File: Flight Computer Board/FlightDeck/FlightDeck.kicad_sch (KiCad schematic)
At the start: 15 parts, among them SW1 SW_SPDT, U1 STM32F205RBT6

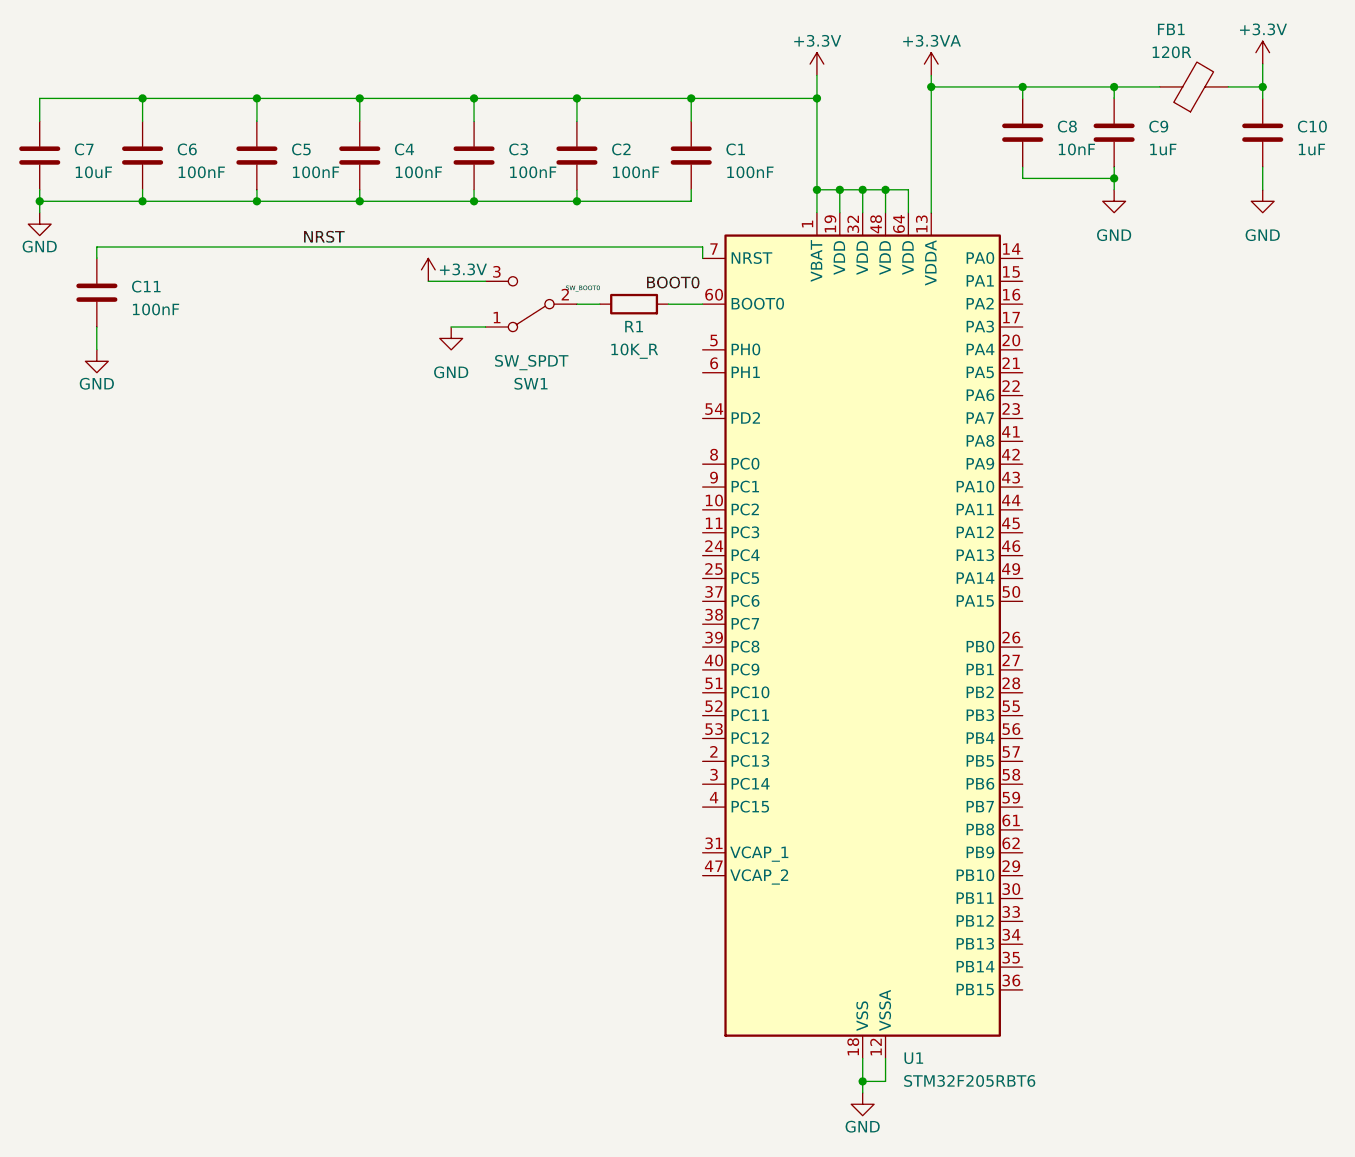
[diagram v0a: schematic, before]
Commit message: fc: init design
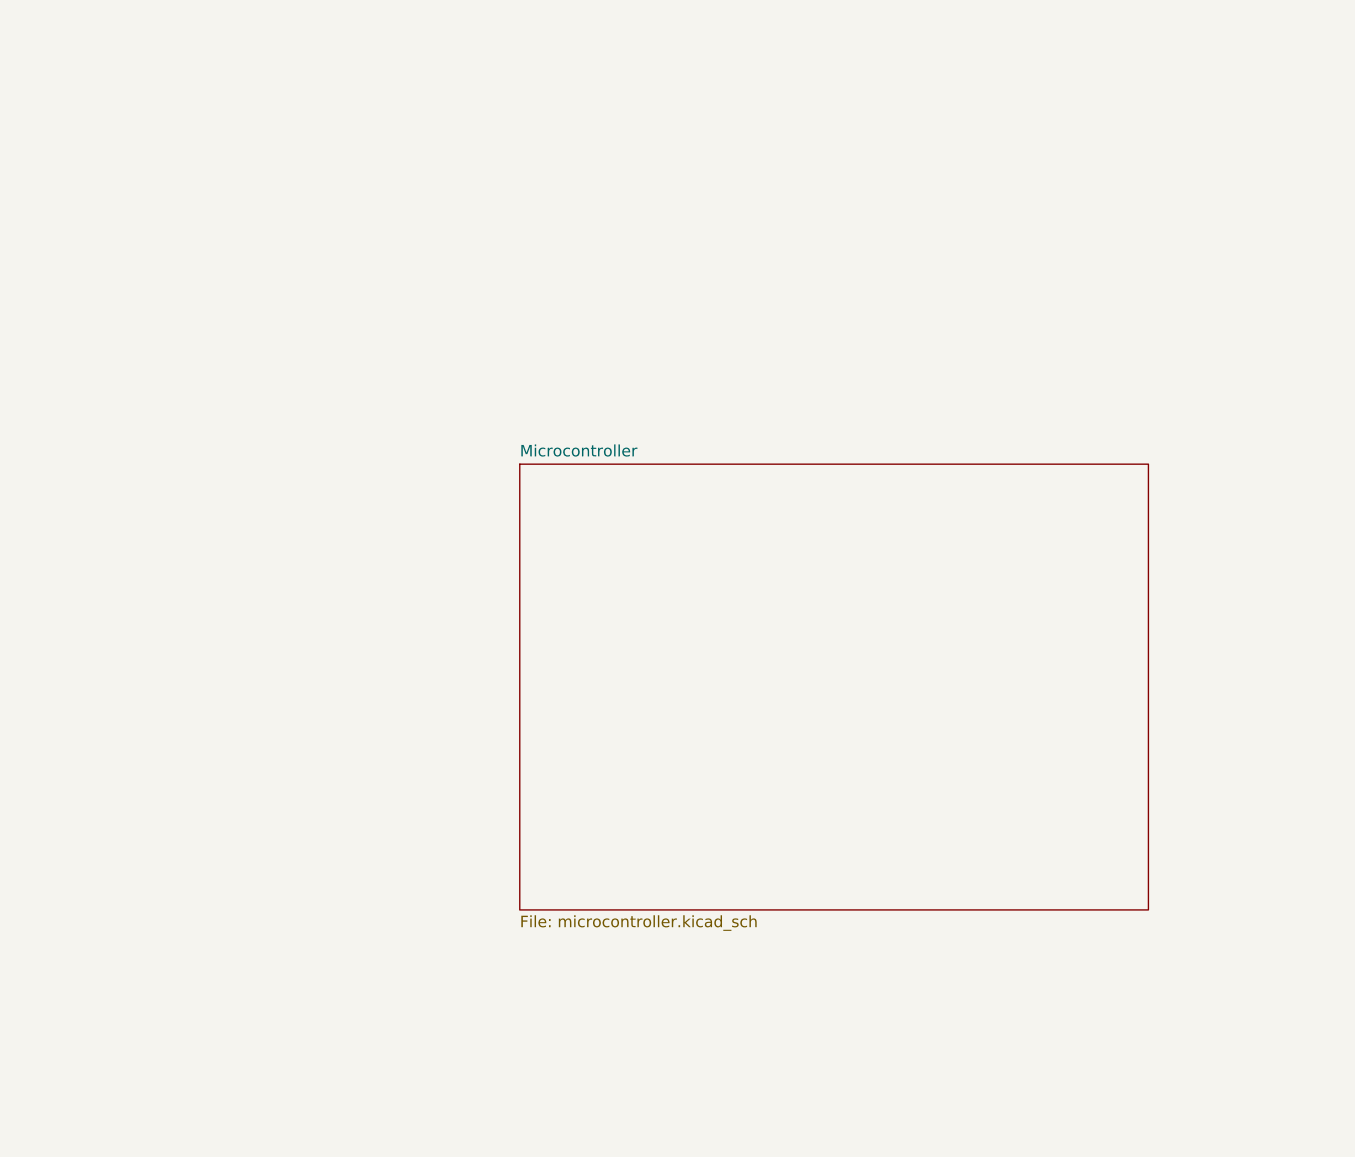
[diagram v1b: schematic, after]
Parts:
- removed C1, C11, C2, C3, C4, C5, C6: 100nF, symbol Device:C
- removed C10, C9: 1uF, symbol Device:C
- removed C7: 10uF, symbol Device:C
- removed C8: 10nF, symbol Device:C
- removed FB1: 120R, symbol Device:FerriteBead
- removed R1: 10K_R, symbol Device:R
- removed SW1: SW_SPDT, symbol Switch:SW_SPDT
- removed U1: STM32F205RBT6, Package_QFP:LQFP-64_10x10mm_P0.5mm, symbol MCU_ST_STM32F2:STM32F205RBTx
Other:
- added sheet Microcontroller (microcontroller.kicad_sch)
